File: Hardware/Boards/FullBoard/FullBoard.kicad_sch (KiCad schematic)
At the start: 20 parts, among them J2 Conn_01x03_Pin, K1 Relay_SPDT, K2 Relay_SPDT, K3 Relay_SPDT, K4 Relay_SPDT, U2 DS18B20-air, U2 DS18B20-water, U4 TEMT6000, U5 GY-8511 UV sensor, U6 Turbidity sensor, U7 Water Level

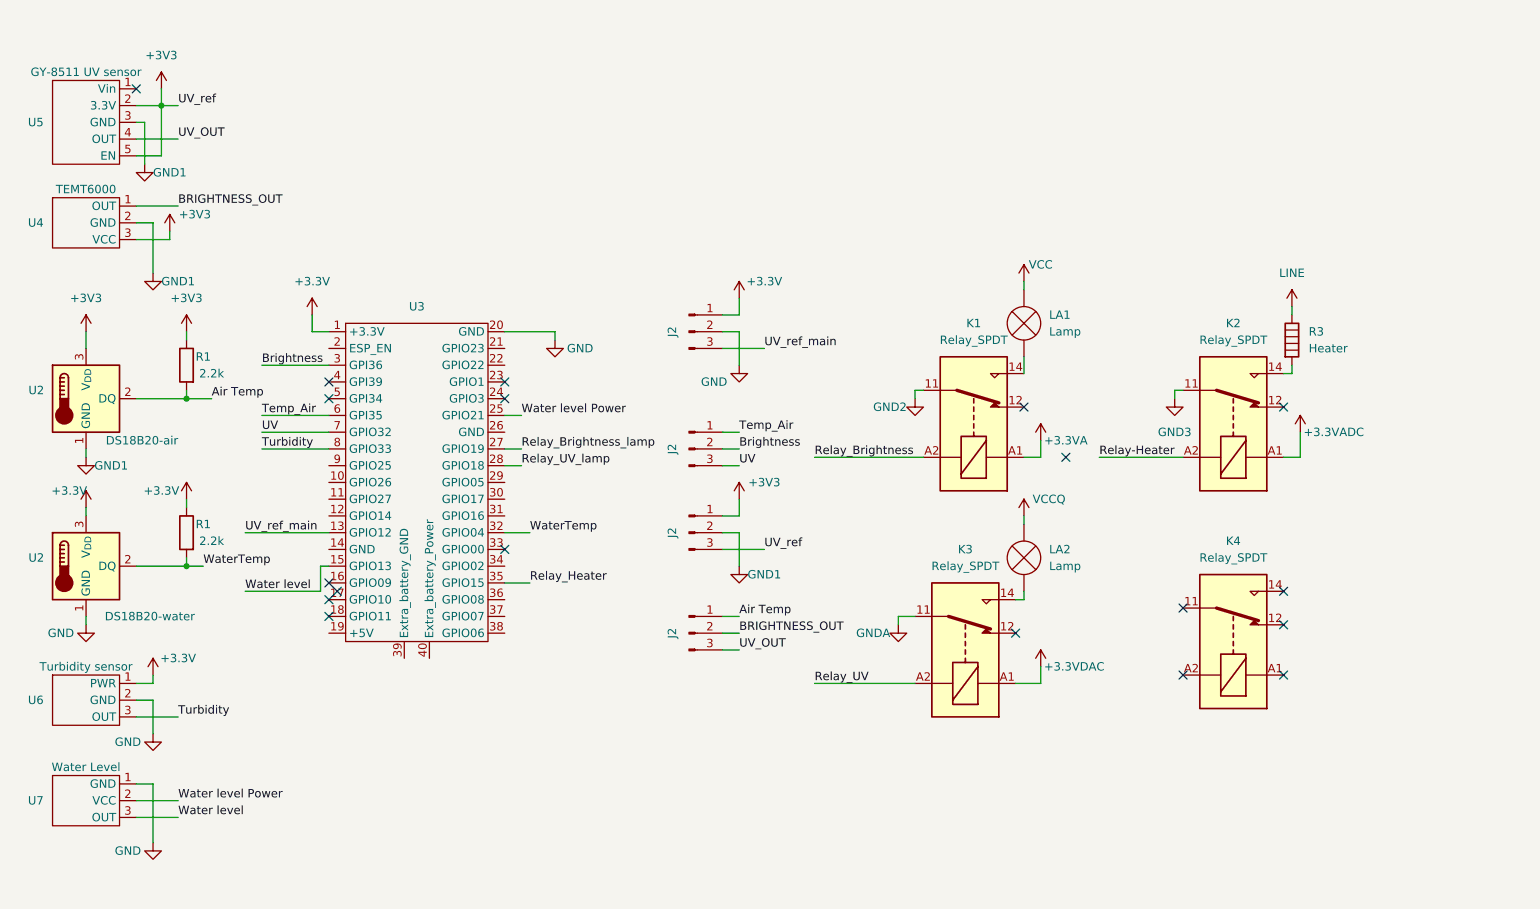
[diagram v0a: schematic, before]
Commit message: Almost completed scheme
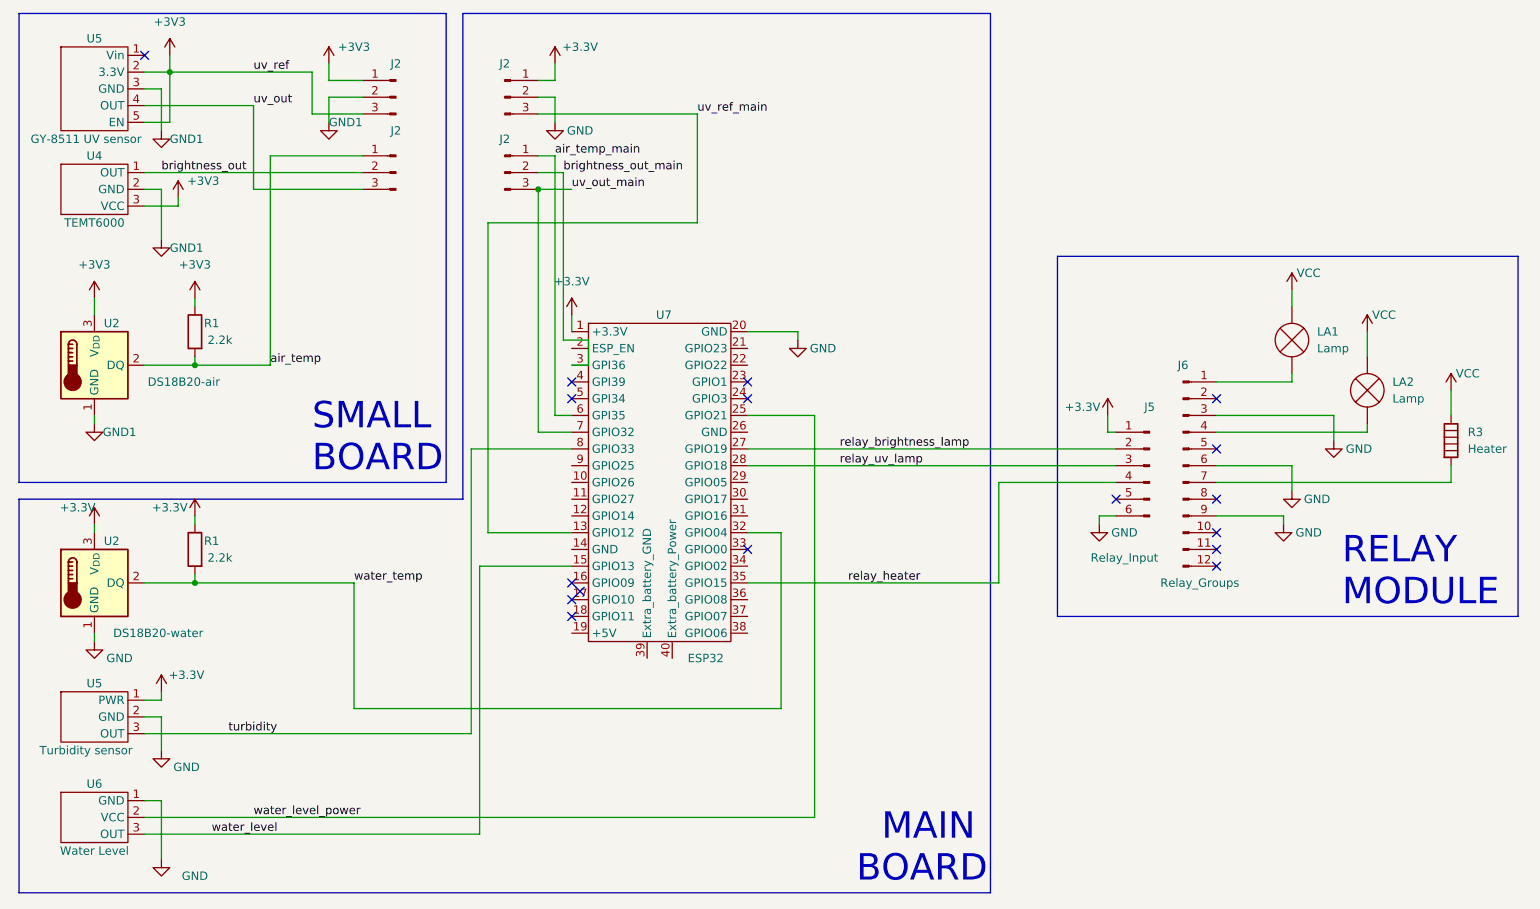
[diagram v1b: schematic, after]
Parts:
- removed J2 (x4): Conn_01x03_Pin, Diplomna:connector_3p, symbol Connector:Conn_01x03_Pin
- removed K1, K2, K3: Relay_SPDT, Diplomna:Relay, symbol Relay:Relay_SPDT
- removed K4: Relay_SPDT, symbol Relay:Relay_SPDT
- removed R1 (x2): 2.2k, Resistor_THT:R_Axial_DIN0204_L3.6mm_D1.6mm_P7.62mm_Horizontal, symbol Device:R
- removed U2: DS18B20-water, Diplomna:DS18B20_3dmodel, symbol Sensor_Temperature:DS18B20
- removed U2: DS18B20-air, Diplomna:DS18B20_3dmodel, symbol Sensor_Temperature:DS18B20
- removed U3: ~, Diplomna:MODULE_ESP32-DEVKITC, symbol Diplomna:olimex-esp32-devkit-lipo-d2
- removed U6: Turbidity sensor, Diplomna:3pin_holes, symbol Diplomna:DFROBOT_-_SEN0189_-_turbidity_sensor
- removed U7: Water Level, Diplomna:3pin_holes, symbol Diplomna:Water_Level_Sensor
- added J2 (x4): Conn_01x03_Pin, Diplomna:connector_3p, symbol Connector:Conn_01x03_Pin
- added J5: Relay_Input, Diplomna:6pin_holes, symbol Connector:Conn_01x06_Pin
- added J6: Relay_Groups, symbol Connector:Conn_01x12_Pin
- added R1 (x2): 2.2k, Resistor_THT:R_Axial_DIN0204_L3.6mm_D1.6mm_P7.62mm_Horizontal, symbol Device:R
- added U2: DS18B20-air, Diplomna:DS18B20_3dmodel, symbol Sensor_Temperature:DS18B20
- added U2: DS18B20-water, Diplomna:DS18B20_3dmodel, symbol Sensor_Temperature:DS18B20
- added U5: Turbidity sensor, Diplomna:3pin_holes, symbol Diplomna:DFROBOT_-_SEN0189_-_turbidity_sensor
- added U6: Water Level, Diplomna:3pin_holes, symbol Diplomna:Water_Level_Sensor
- added U7: ESP32, symbol Diplomna:olimex-esp32-devkit-lipo-d2
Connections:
- net LINE is gone; now on net VCC: R3.1
- net VCCQ is gone; now on net VCC: LA2.2 (+)
- net +3.3V: now also J2.1 (Pin_1), J5.1 (Pin_1), R1.1, U2.3 (V_{DD}), U5.1 (PWR), U7.1 (+3.3V)
- net +3V3: now also J2.1 (Pin_1), J2.3 (Pin_3), R1.1, U2.3 (V_{DD})
- net GND: now also J2.2 (Pin_2), J5.6 (Pin_6), J6.3 (Pin_3), J6.6 (Pin_6), J6.9 (Pin_9), U2.1 (GND), U5.2 (GND), U6.1 (GND), U7.20 (GND)
- net GND1: now also J2.2 (Pin_2), U2.1 (GND)
- net at LA2.1 (-): now also J6.4 (Pin_4)
- net at LA1.1 (-): now also J6.1 (Pin_1)
- net at R3.2: now also J6.7 (Pin_7)
- net BRIGHTNESS_OUT renamed brightness_out
- net brightness_out: now also J2.2 (Pin_2)
- net UV_OUT renamed uv_out
- net uv_out: now also J2.3 (Pin_3)
- new net air_temp: J2.1 (Pin_1), R1.2, U2.2 (DQ)
- new net air_temp_main: J2.1 (Pin_1), U7.6 (GPI35)
- new net brightness_out_main: J2.2 (Pin_2), U7.3 (GPI36)
- new net relay_brightness_lamp: J5.2 (Pin_2), U7.27 (GPIO19)
- new net relay_heater: J5.4 (Pin_4), U7.35 (GPIO15)
- new net relay_uv_lamp: J5.3 (Pin_3), U7.28 (GPIO18)
- new net turbidity: U5.3 (OUT), U7.8 (GPIO33)
- new net uv_out_main: J2.3 (Pin_3), U7.7 (GPIO32)
- new net uv_ref_main: J2.3 (Pin_3), U7.13 (GPIO12)
- new net water_level: U6.3 (OUT), U7.15 (GPIO13)
- new net water_level_power: U6.2 (VCC), U7.25 (GPIO21)
- new net water_temp: R1.2, U2.2 (DQ), U7.32 (GPIO04)
- no-connect marks 19 -> 17
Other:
- note added: "BOARD"
- note added: "MAIN"
- note added: "MODULE"
- note added: "RELAY"
- note added: "SMALL"
